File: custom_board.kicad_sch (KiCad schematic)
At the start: 4 parts, among them IC1 TMPM46BF10FG

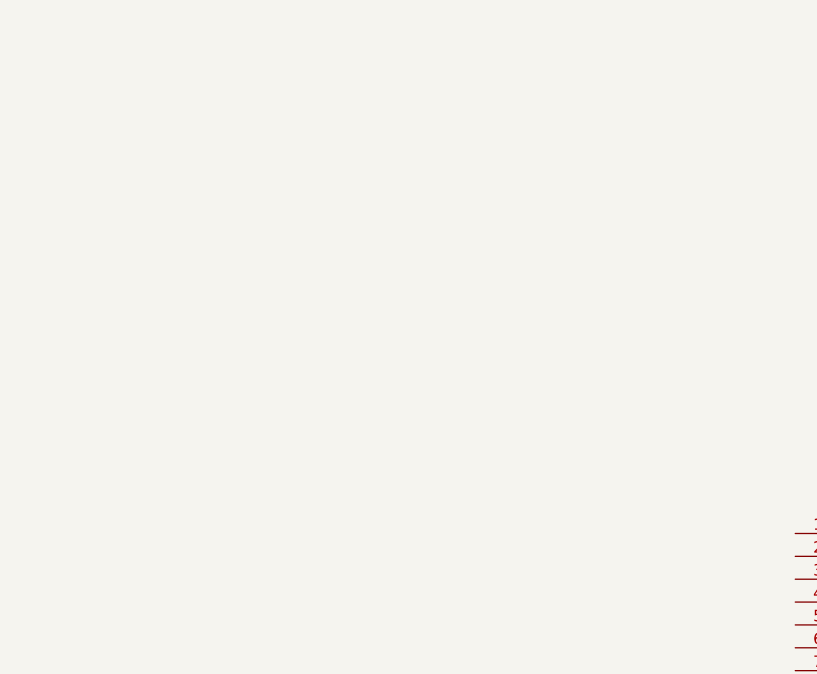
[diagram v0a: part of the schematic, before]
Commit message: working on pin connections
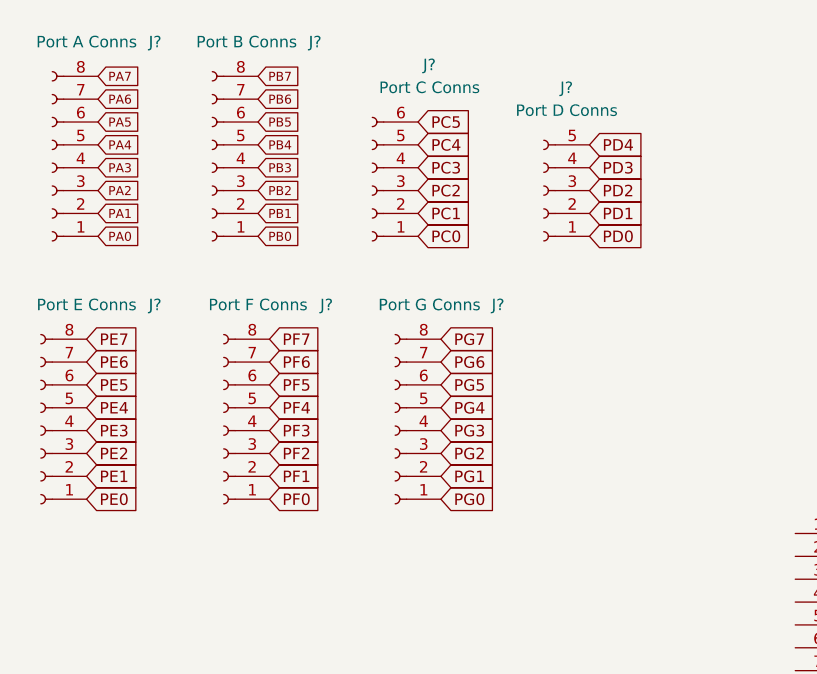
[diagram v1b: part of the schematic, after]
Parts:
- added J?: Port A Conns, symbol Connector:Conn_01x08_Female
- added J?: Port C Conns, symbol Connector:Conn_01x06_Female
- added J?: Port F Conns, symbol Connector:Conn_01x08_Female
- added J?: Port G Conns, symbol Connector:Conn_01x08_Female
- added J?: Port B Conns, symbol Connector:Conn_01x08_Female
- added J?: Port D Conns, symbol Connector:Conn_01x05_Female
- added J?: Port E Conns, symbol Connector:Conn_01x08_Female
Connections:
- new net PA0: J?.1 (Pin_1)
- new net PA1: J?.2 (Pin_2)
- new net PA2: J?.3 (Pin_3)
- new net PA3: J?.4 (Pin_4)
- new net PA4: J?.5 (Pin_5)
- new net PA5: J?.6 (Pin_6)
- new net PA6: J?.7 (Pin_7)
- new net PA7: J?.8 (Pin_8)
- new net PB0: J?.1 (Pin_1)
- new net PB1: J?.2 (Pin_2)
- new net PB2: J?.3 (Pin_3)
- new net PB3: J?.4 (Pin_4)
- new net PB4: J?.5 (Pin_5)
- new net PB5: J?.6 (Pin_6)
- new net PB6: J?.7 (Pin_7)
- new net PB7: J?.8 (Pin_8)
- new net PC0: J?.1 (Pin_1)
- new net PC1: J?.2 (Pin_2)
- new net PC2: J?.3 (Pin_3)
- new net PC3: J?.4 (Pin_4)
- new net PC4: J?.5 (Pin_5)
- new net PC5: J?.6 (Pin_6)
- new net PD0: J?.1 (Pin_1)
- new net PD1: J?.2 (Pin_2)
- new net PD2: J?.3 (Pin_3)
- new net PD3: J?.4 (Pin_4)
- new net PD4: J?.5 (Pin_5)
- new net PE0: J?.1 (Pin_1)
- new net PE1: J?.2 (Pin_2)
- new net PE2: J?.3 (Pin_3)
- new net PE3: J?.4 (Pin_4)
- new net PE4: J?.5 (Pin_5)
- new net PE5: J?.6 (Pin_6)
- new net PE6: J?.7 (Pin_7)
- new net PE7: J?.8 (Pin_8)
- new net PF0: J?.1 (Pin_1)
- new net PF1: J?.2 (Pin_2)
- new net PF2: J?.3 (Pin_3)
- new net PF3: J?.4 (Pin_4)
- new net PF4: J?.5 (Pin_5)
- new net PF5: J?.6 (Pin_6)
- new net PF6: J?.7 (Pin_7)
- new net PF7: J?.8 (Pin_8)
- new net PG0: J?.1 (Pin_1)
- new net PG1: J?.2 (Pin_2)
- new net PG2: J?.3 (Pin_3)
- new net PG3: J?.4 (Pin_4)
- new net PG4: J?.5 (Pin_5)
- new net PG5: J?.6 (Pin_6)
- new net PG6: J?.7 (Pin_7)
- new net PG7: J?.8 (Pin_8)
